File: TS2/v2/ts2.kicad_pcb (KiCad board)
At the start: 2 copper layers, 100 parts, among them P1 FTDI (TERMINAL), P2 FTDI (HOST), P3 +5V POWER, SW1 RESET, SW2 SINGLE STEP/RUN, SW3 STEP, SW4 ABORT, SW5 POWER, U1 555, U10 74LS32, U11 HM6264, U12 28C64, U13 HM6264, U14 28C64, U15 HM6264, U16 28C64, U17 HM6264, U18 28C64, U19 74LS20, U2 8 MHz, U20 74LS74, U21 74LS161, U22 74LS161, U23 74LS74, U24 74LS260, U25 74LS260, U26 74LS138, U27 25LS2548, U28 74LS148, U29 6850, U3 74LS00, U30 6850, U31 MC14411, U32 74LS138, U33 74LS138, U34 74LS00, U35 74LS74, U4 74LS06, U5 74LS04, U6 68000, U7 74LS08, U8 74LS32, U9 74LS32, Y1 1.842MHz

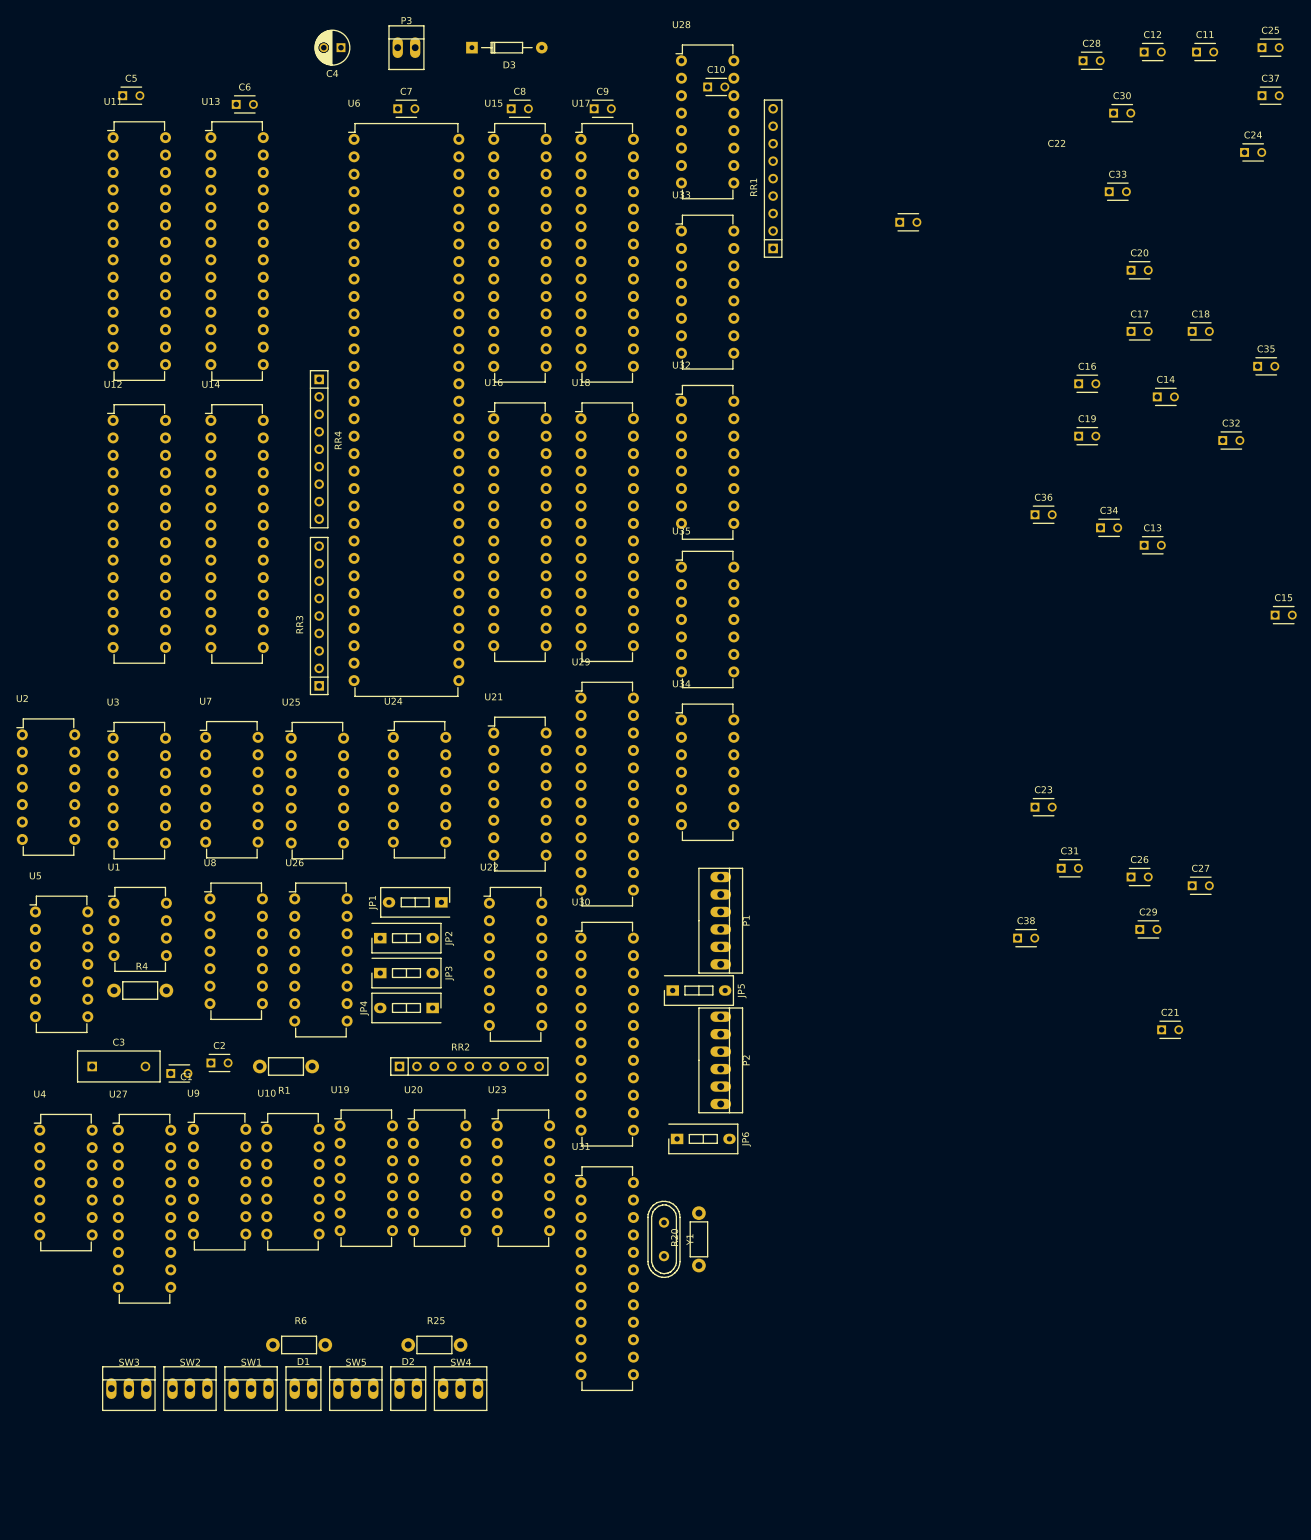
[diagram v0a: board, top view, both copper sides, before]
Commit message: Working on PCB layout.
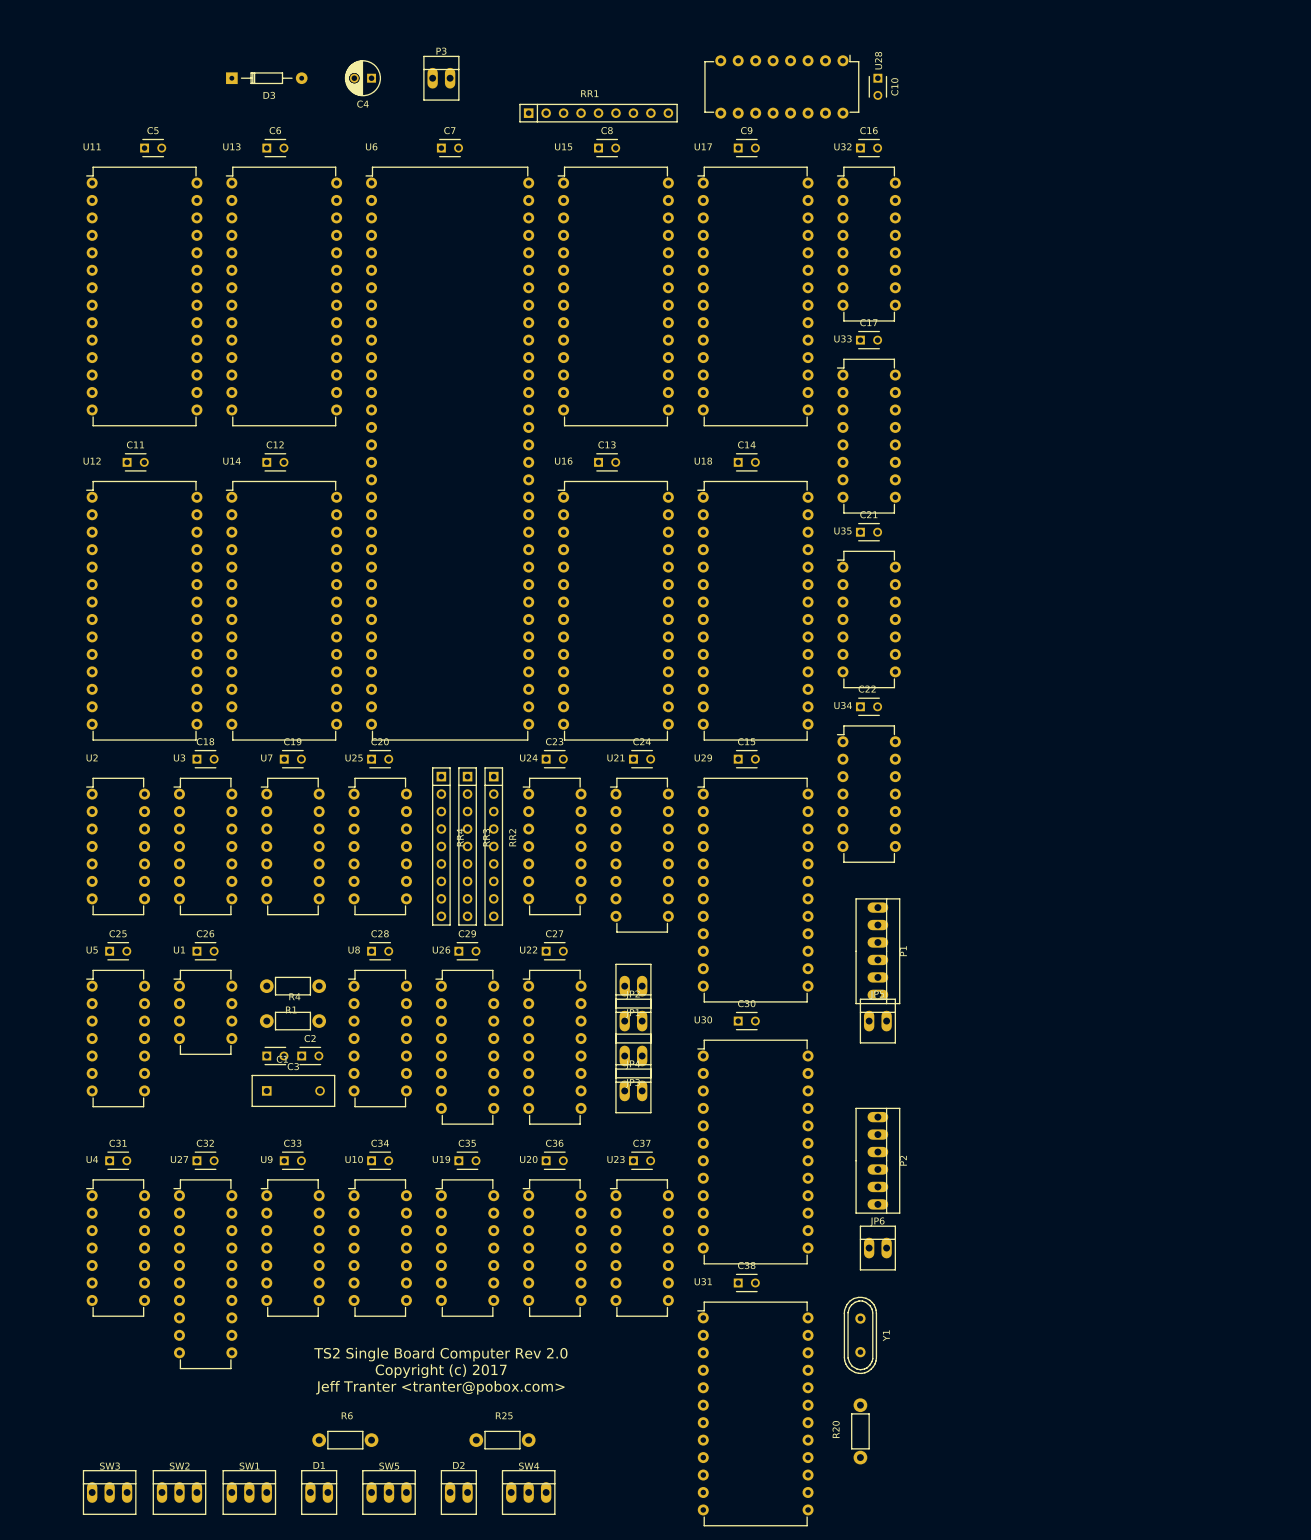
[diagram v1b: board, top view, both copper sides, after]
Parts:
- JP1, JP2, JP3, JP4, JP5, JP6: footprint Buttons_Switches_ThroughHole:SW_DIP_x1_Slide -> Connect:PINHEAD1-2
- U11, U12, U13, U14, U15, U16, U17, U18: footprint Housings_DIP:DIP-28_W7.62mm -> Housings_DIP:DIP-28_W15.24mm
- U29, U30, U31: footprint Housings_DIP:DIP-24_W7.62mm -> Housings_DIP:DIP-24_W15.24mm
- U6: footprint Housings_DIP:DIP-64_W15.24mm -> Housings_DIP:DIP-64_W22.86mm
- moved C25 213.0 mm to (30.5, 149.9)
- moved C33 185.1 mm to (55.9, 180.3)
- moved C32 182.3 mm to (43.2, 180.3)
- moved C37 179.9 mm to (106.7, 180.3)
- moved C11 166.6 mm to (33.0, 78.7)
- moved C28 165.8 mm to (68.6, 149.9)
- moved C35 163.9 mm to (81.3, 180.3)
- moved C18 157.6 mm to (43.2, 121.9)
- moved C31 144.8 mm to (30.5, 180.3)
- moved C30 142.9 mm to (121.9, 160.0)
- moved C12 140.9 mm to (53.3, 78.7)
- moved C34 140.4 mm to (68.6, 180.3)
- moved C26 136.3 mm to (43.2, 149.9)
- moved C20 131.4 mm to (68.6, 121.9)
- moved C24 125.3 mm to (106.7, 121.9)
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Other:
- board text added: "TS2 Single Board Computer Rev 2.0 Copyright (c) 2017 Jeff Tranter <tranter@pobox.com>"
